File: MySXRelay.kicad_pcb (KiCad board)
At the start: 2 copper layers, 47.2 x 45.1 mm, 51 parts, among them K1 FH44L-1AT-L1-DC5V, Q1 2N7002, U1 MIC4427, U2 BL0942, U3 BP2525X, U4 Si8642BB-B-IS1, U5 MCP1703Ax-180xxTT

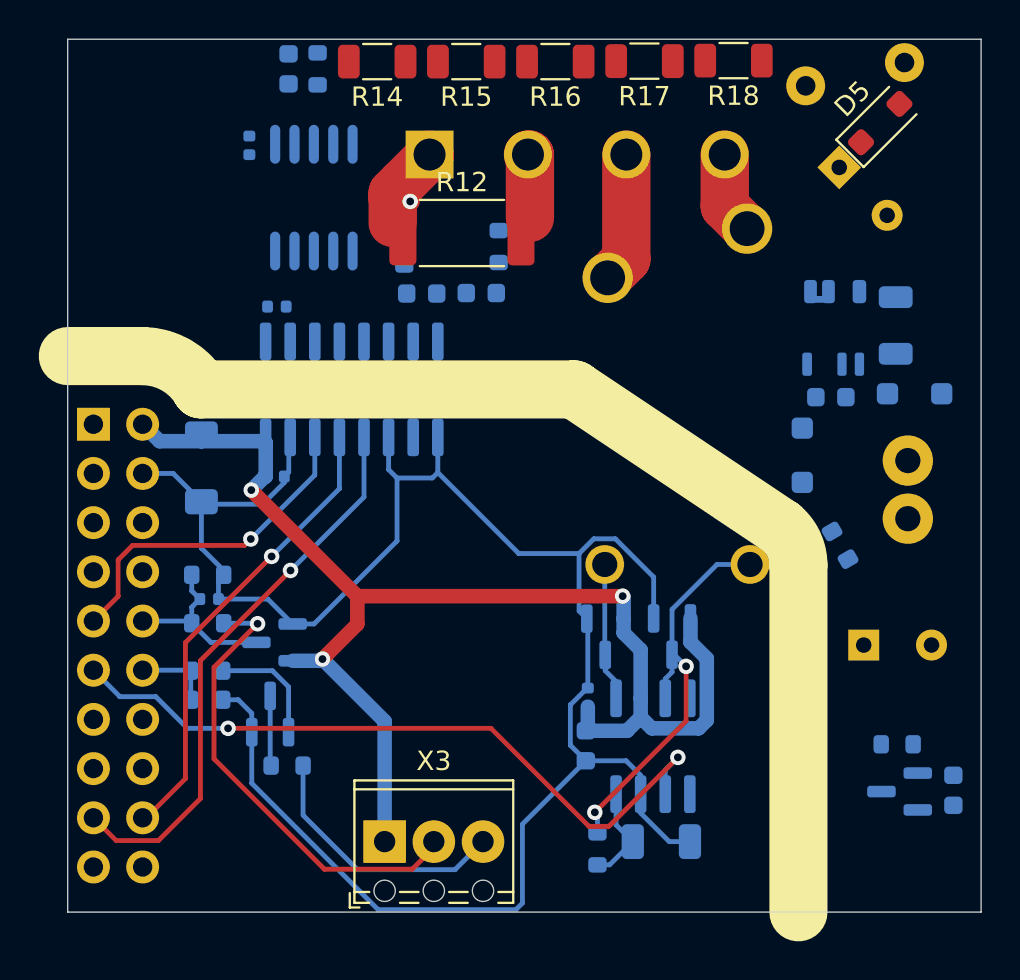
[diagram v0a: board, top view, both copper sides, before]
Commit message: WIP PCB
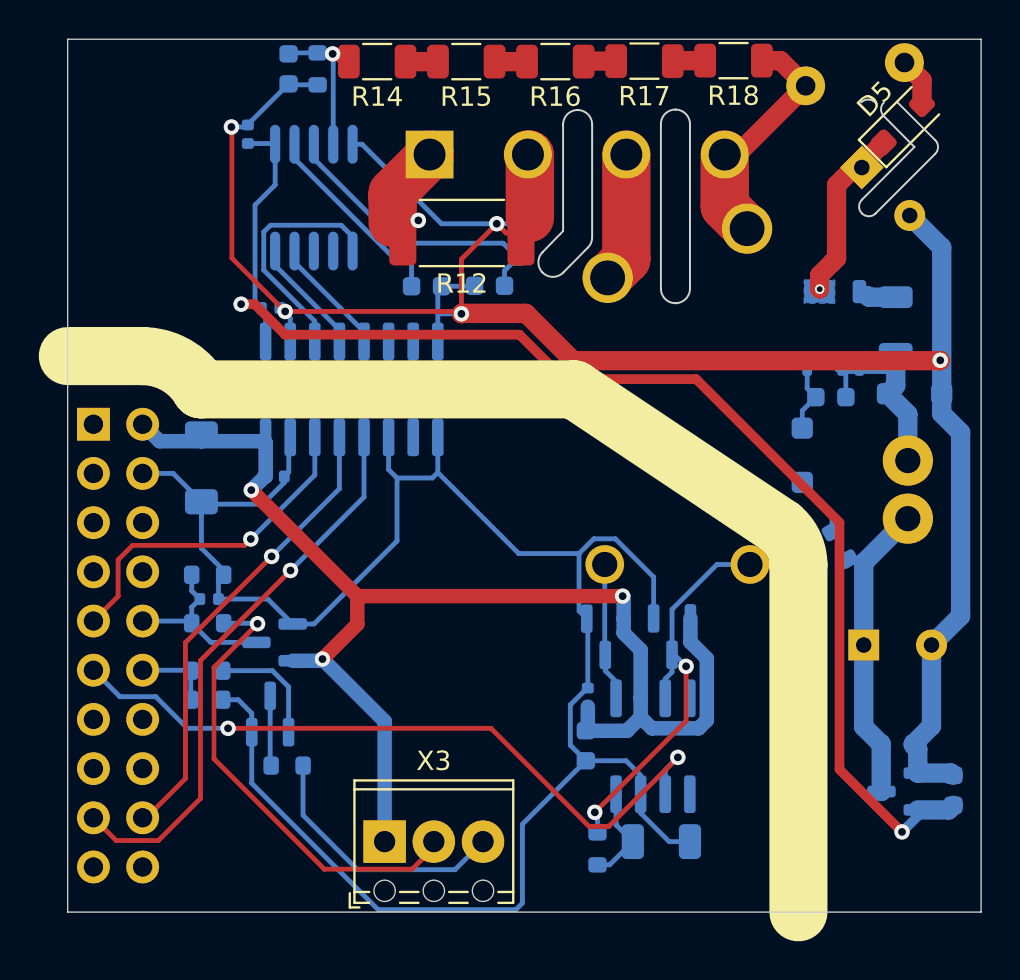
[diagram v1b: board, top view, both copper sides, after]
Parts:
- moved R11 5.86 mm to (158.7, 92.9)
- moved R10 4.86 mm to (152.8, 92.9)
- moved C5 1.17 mm to (176.4, 89.1)
- moved D5 1.17 mm to (178.5, 86.8)
- moved C9 0.58 mm to (144.7, 87.4), turned to 90 degrees
- moved C11 0.57 mm to (157.2, 95.2)
- moved C10 0.45 mm to (153.9, 95.2)
- moved C13 0.33 mm to (145.9, 96.3)
- turned R12 to 180 degrees
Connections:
- X2 pad 1: N_IN -> N_OUT
- X2 pad 2: N_OUT -> N_IN
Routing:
- net N_IN: track 6.84 -> 113.2 mm, vias 1 -> 5
- net +3V3: track 0.00 -> 69.3 mm, vias 0 -> 2
- net Net-(U5-VI): track 0.00 -> 16.3 mm
- net Net-(U2-IN): track 0.00 -> 15.1 mm
- net CF1: track 0.00 -> 12.5 mm
- net Net-(D6-K): track 0.00 -> 10.9 mm
- net Net-(U2-IP): track 0.00 -> 10.2 mm
- net Net-(D5-K): track 0.00 -> 10.1 mm, vias 0 -> 1
- net L_IN: track 4.30 -> 12.8 mm
- net Net-(U2-VP): track 0.00 -> 8.00 mm, vias 0 -> 1
- net RX: track 0.00 -> 6.15 mm
- net TX: track 0.00 -> 6.04 mm
- net Net-(D7-K): track 0.00 -> 3.78 mm
- net Net-(D7-A): track 0.00 -> 3.17 mm
- net Net-(D5-A): track 0.00 -> 2.52 mm
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- added copper zone on B.Cu, net Net-(D5-K)
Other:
- outline, holes or cut-outs redrawn
